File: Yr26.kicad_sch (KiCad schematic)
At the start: 0 parts

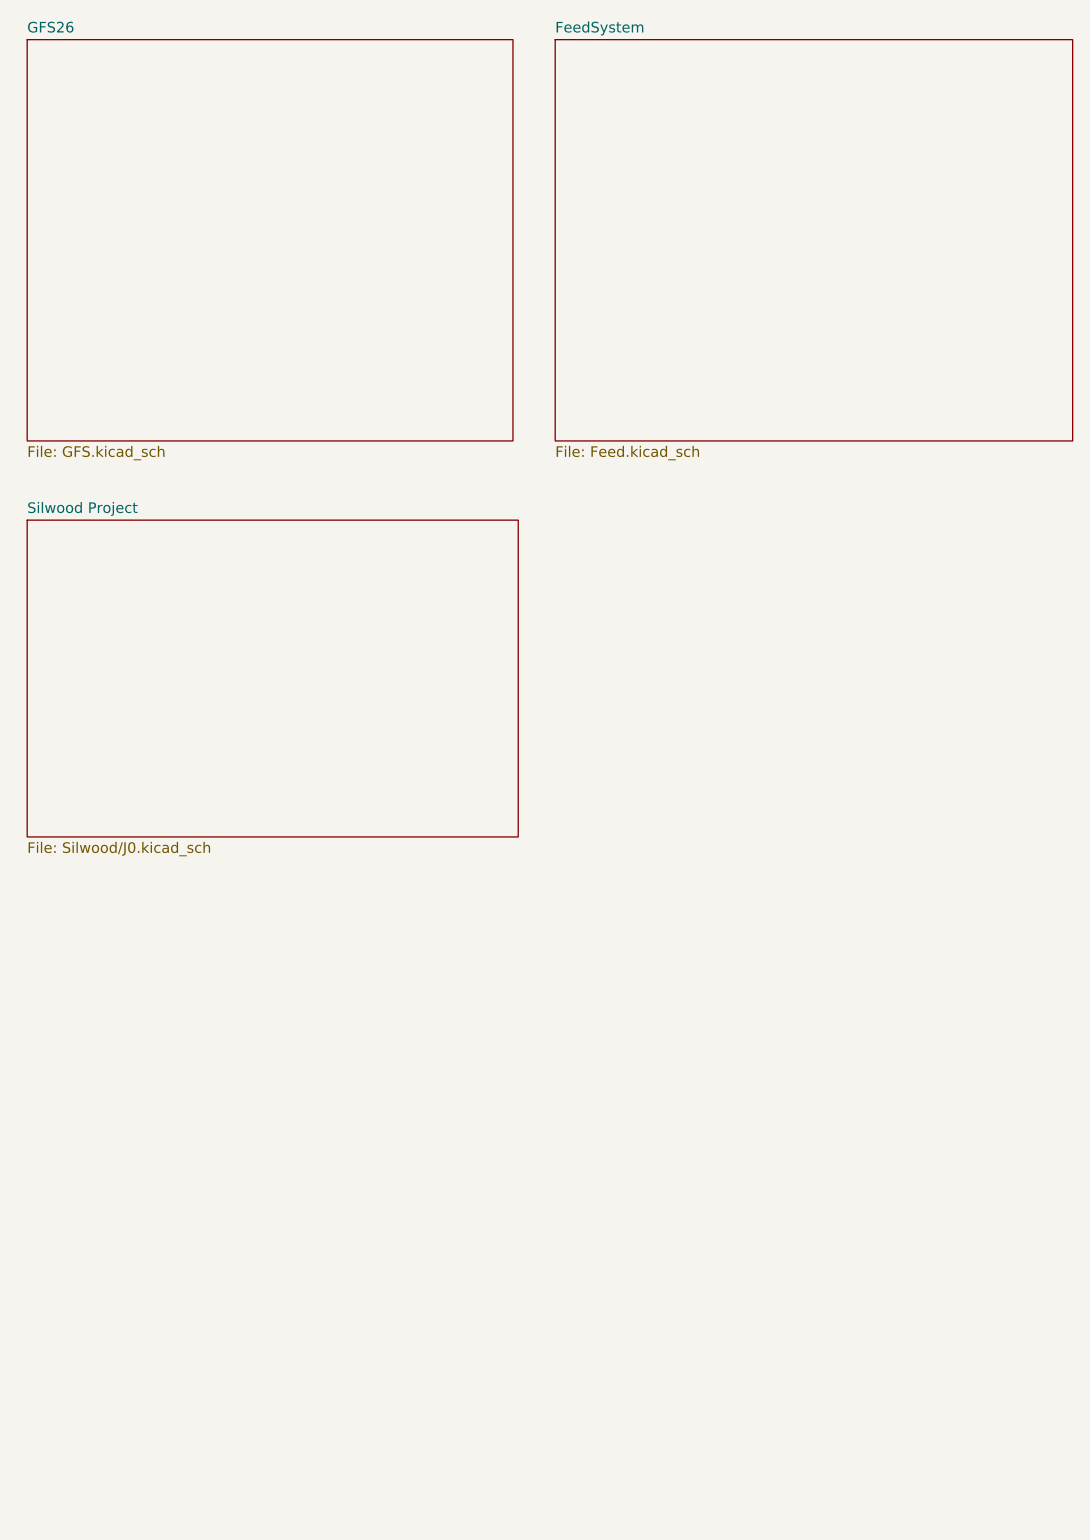
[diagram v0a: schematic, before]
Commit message: j0
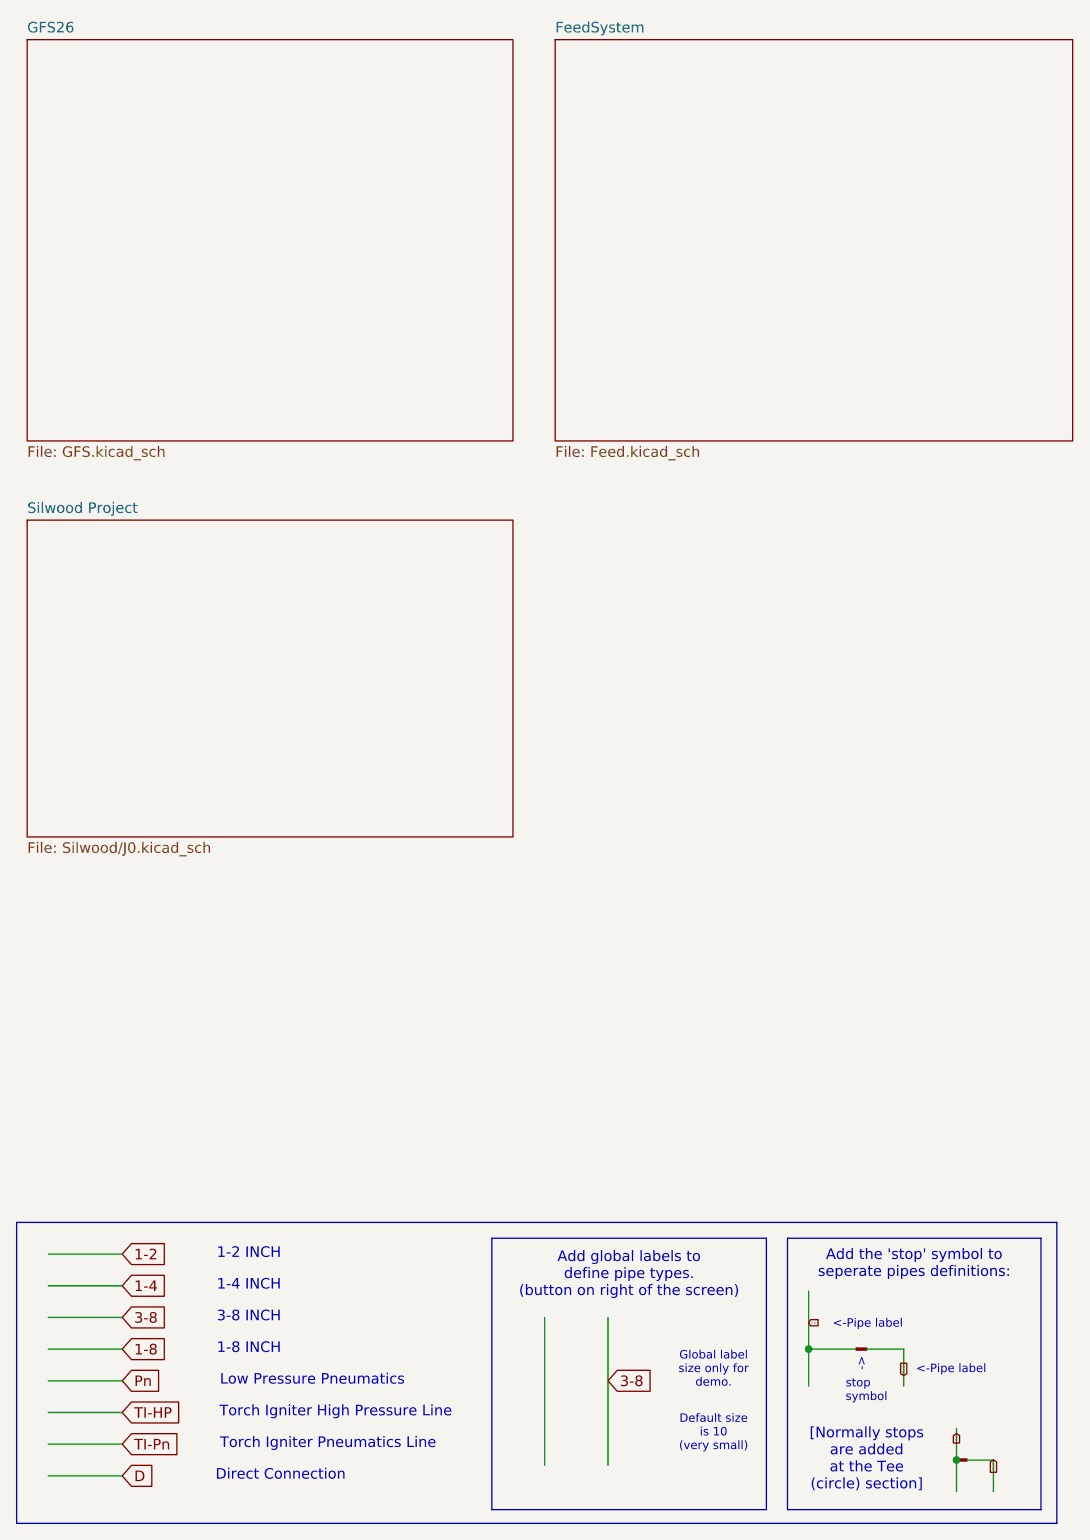
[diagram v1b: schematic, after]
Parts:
- added U3, U4: ~, symbol PID_symbols:stop
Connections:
- new net 1-2: U3., U4.
- new net TI-HP: U3., U4.
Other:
- note added: "->"
- note added: "1-2 INCH"
- note added: "1-4 INCH"
- note added: "1-8 INCH"
- note added: "3-8 INCH"
- note added: "<-Pipe label"
- note added: "Add global labels to define pipe types. (button on right of the screen)"
- note added: "Add the 'stop' symbol to seperate pipes definitions:"
- note added: "Default size is 10 (very small)"
- note added: "Direct Connection"
- note added: "Global label size only for demo."
- note added: "Low Pressure Pneumatics"
- note added: "Torch Igniter High Pressure Line"
- note added: "Torch Igniter Pneumatics Line"
- note added: "[Normally stops are added at the Tee (circle) section]"
- note added: "stop symbol"

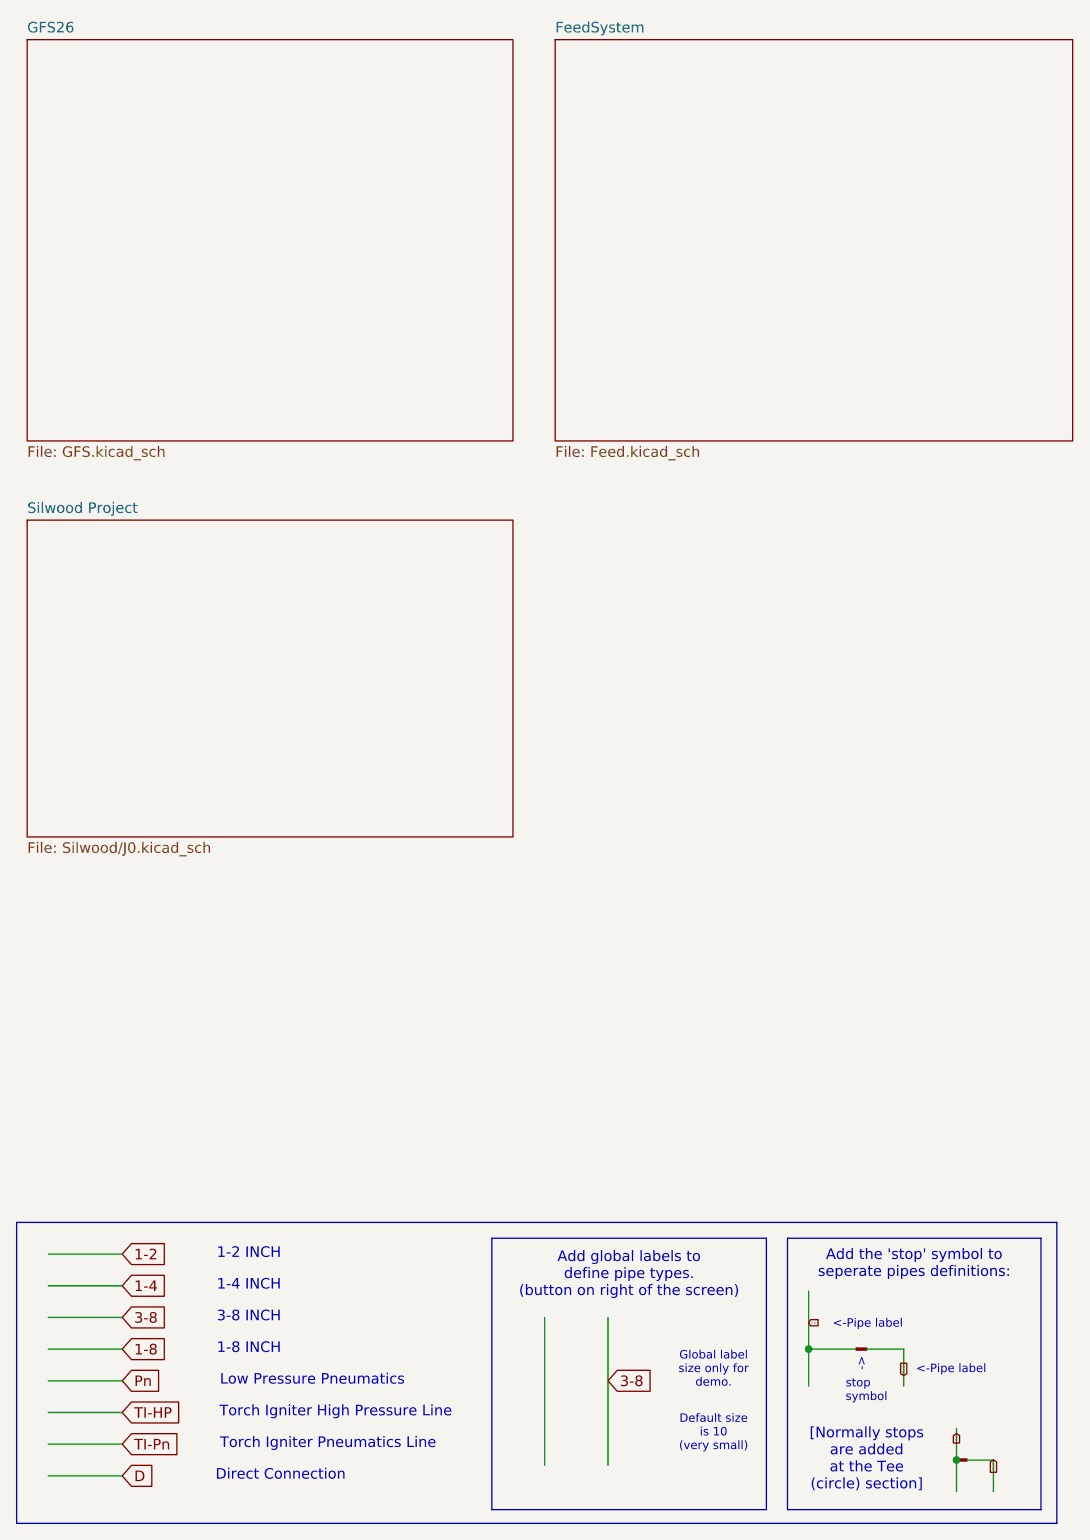
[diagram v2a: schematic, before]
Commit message: Formatiing
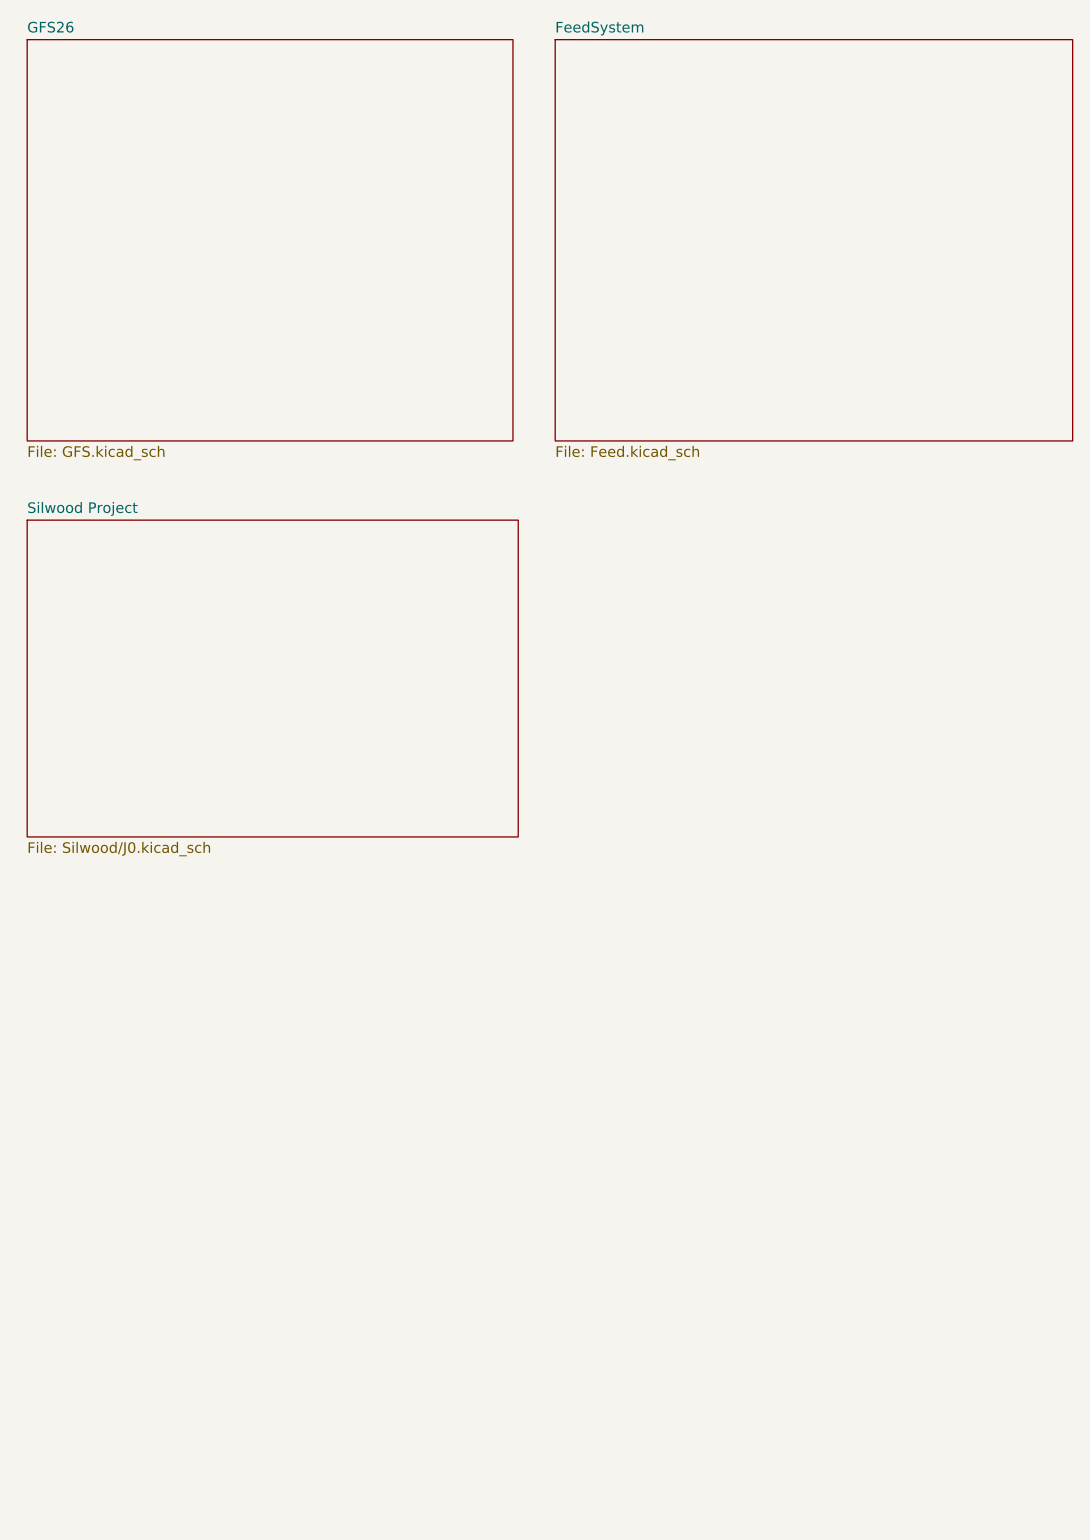
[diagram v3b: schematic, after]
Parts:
- removed U3, U4: ~, symbol PID_symbols:stop
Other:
- note removed: "->"
- note removed: "1-2 INCH"
- note removed: "1-4 INCH"
- note removed: "1-8 INCH"
- note removed: "3-8 INCH"
- note removed: "<-Pipe label"
- note removed: "Add global labels to define pipe types. (button on right of the screen)"
- note removed: "Add the 'stop' symbol to seperate pipes definitions:"
- note removed: "Default size is 10 (very small)"
- note removed: "Direct Connection"
- note removed: "Global label size only for demo."
- note removed: "Low Pressure Pneumatics"
- note removed: "Torch Igniter High Pressure Line"
- note removed: "Torch Igniter Pneumatics Line"
- note removed: "[Normally stops are added at the Tee (circle) section]"
- note removed: "stop symbol"
